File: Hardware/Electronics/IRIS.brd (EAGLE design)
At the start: 74 x 15.6 mm, 21 parts, among them U1 AT32UC3C, U2 TCD1304AP, X2 MINI-USB-32005-201

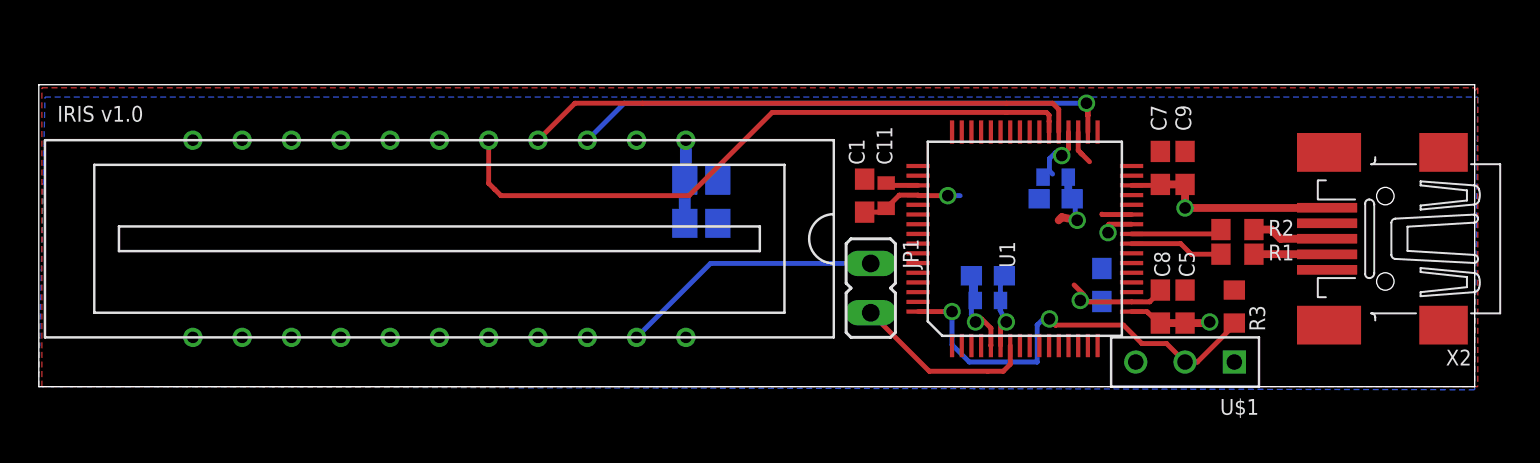
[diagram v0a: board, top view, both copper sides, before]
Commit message: First candidate for v1.0
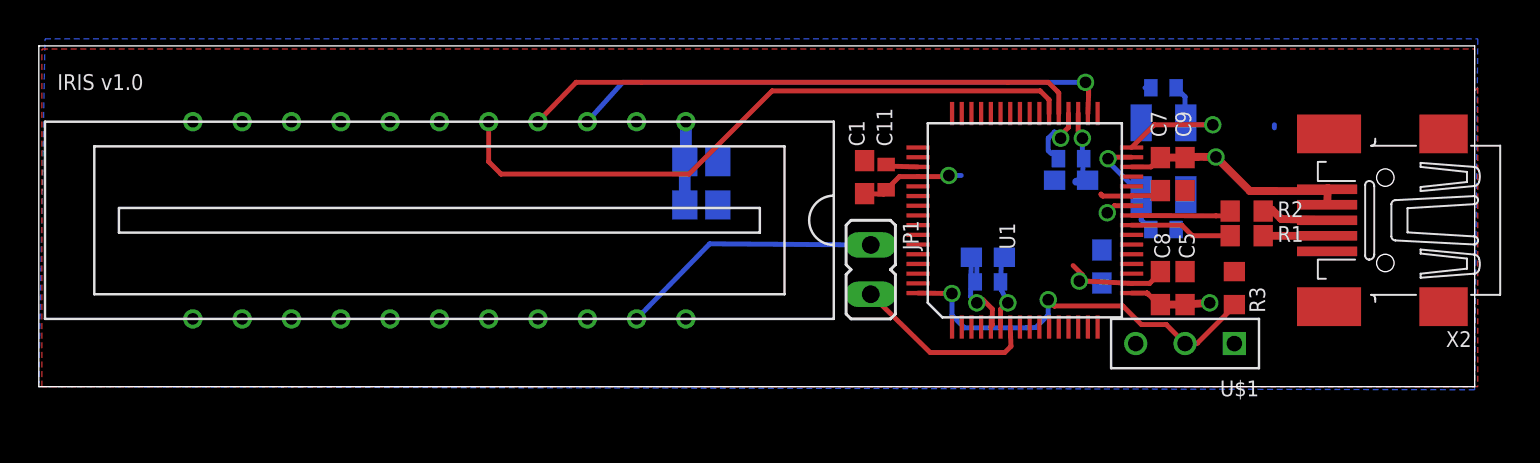
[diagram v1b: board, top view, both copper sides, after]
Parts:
- added C12, C13: 22pF, rcl:C0402
- added Q2: 12MHz, Forrequi:CRYSTAL-SMD-5X3
- JP1: value (none) -> Output signal
- moved C3 1.24 mm to (53.2, 10.6)
- moved C4 1.24 mm to (53.2, 11.7)
- moved R2 1.06 mm to (62.2, 9.05)
- moved R1 1.06 mm to (62.2, 7.78)
- moved C1 0.95 mm to (42.5, 10.8)
- moved C10 0.95 mm to (54.8, 6.19)
- moved C11 0.95 mm to (43.7, 10.8)
- moved C17 0.95 mm to (34.1, 9.37)
- moved C6 0.95 mm to (48.9, 6.67)
- moved U$1 0.95 mm to (59.1, 3.49)
- moved C2 0.95 mm to (48.9, 5.40)
- moved C5 0.95 mm to (59.1, 5.08)
- moved C8 0.95 mm to (57.8, 5.08)
- moved JP1 0.95 mm to (42.9, 6.03)
- moved R3 0.95 mm to (61.6, 5.08)
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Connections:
- removed net TCK: U1.P$1
- removed net TDI: U1.P$2
- removed net TDO: U1.P$3
- removed net TMS: U1.P$4
- removed net VAD: U2.P$2
- removed net VDD: C17.1, C18.1, U2.P$1
- removed net XIN0: U1.P$31
- removed net XOUT0: U1.P$32
- new net N$21: C12.1, Q2.3, U1.P$31
- new net N$22: C13.1, Q2.1, U1.P$32
- net GND: now also C12.2, C13.2
- net VCC: now also C17.1, C18.1, U2.P$1, U2.P$2
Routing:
- net N$22: track 0.00 -> 8.53 mm, vias 0 -> 1
- net VCC: track 21.5 -> 27.8 mm
- net N$21: track 0.00 -> 5.81 mm, vias 0 -> 1
- net VDD: track 4.31 -> 0.00 mm
- net GND: track 29.6 -> 33.4 mm
- net RSTN: track 23.1 -> 21.5 mm
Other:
- board size 74 x 15.6 mm -> 74 x 17.6 mm
